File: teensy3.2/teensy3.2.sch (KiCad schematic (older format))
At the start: 80 parts, among them J2 USB_B_Micro, SW1 Prog, U1 LP38691SD-3.3, U2 MKL02Z32VFG4, U3 MK20DX256VLH7, Y1 32.768 KHz, Y2 16 MHz

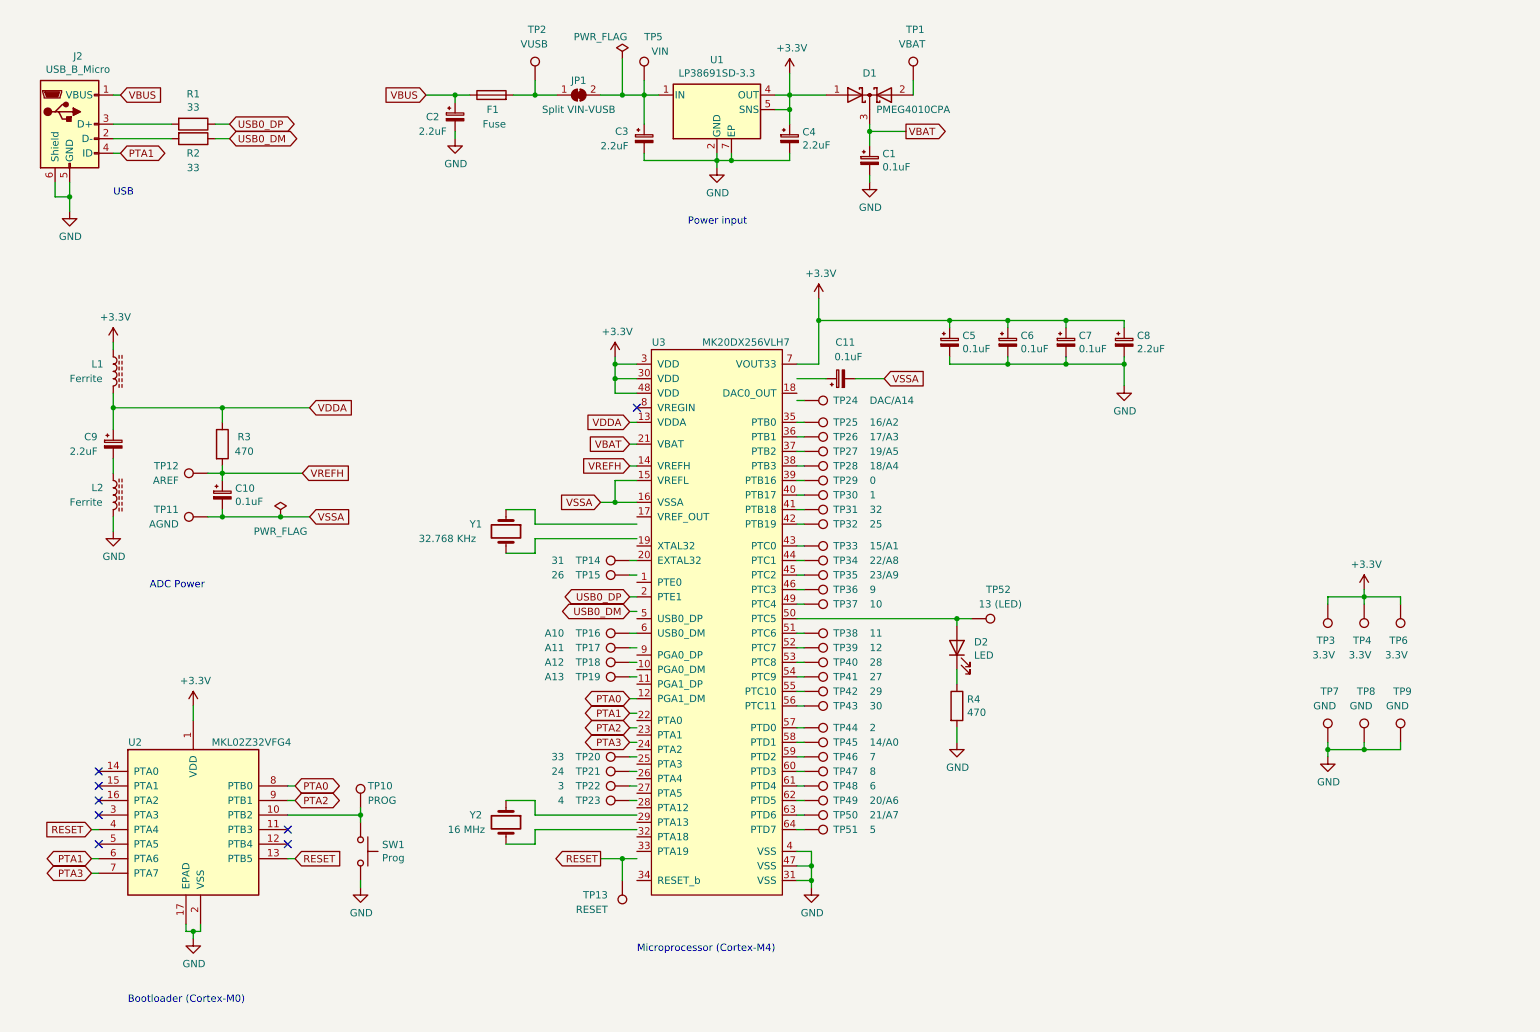
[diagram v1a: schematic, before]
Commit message: avances sch + pcb
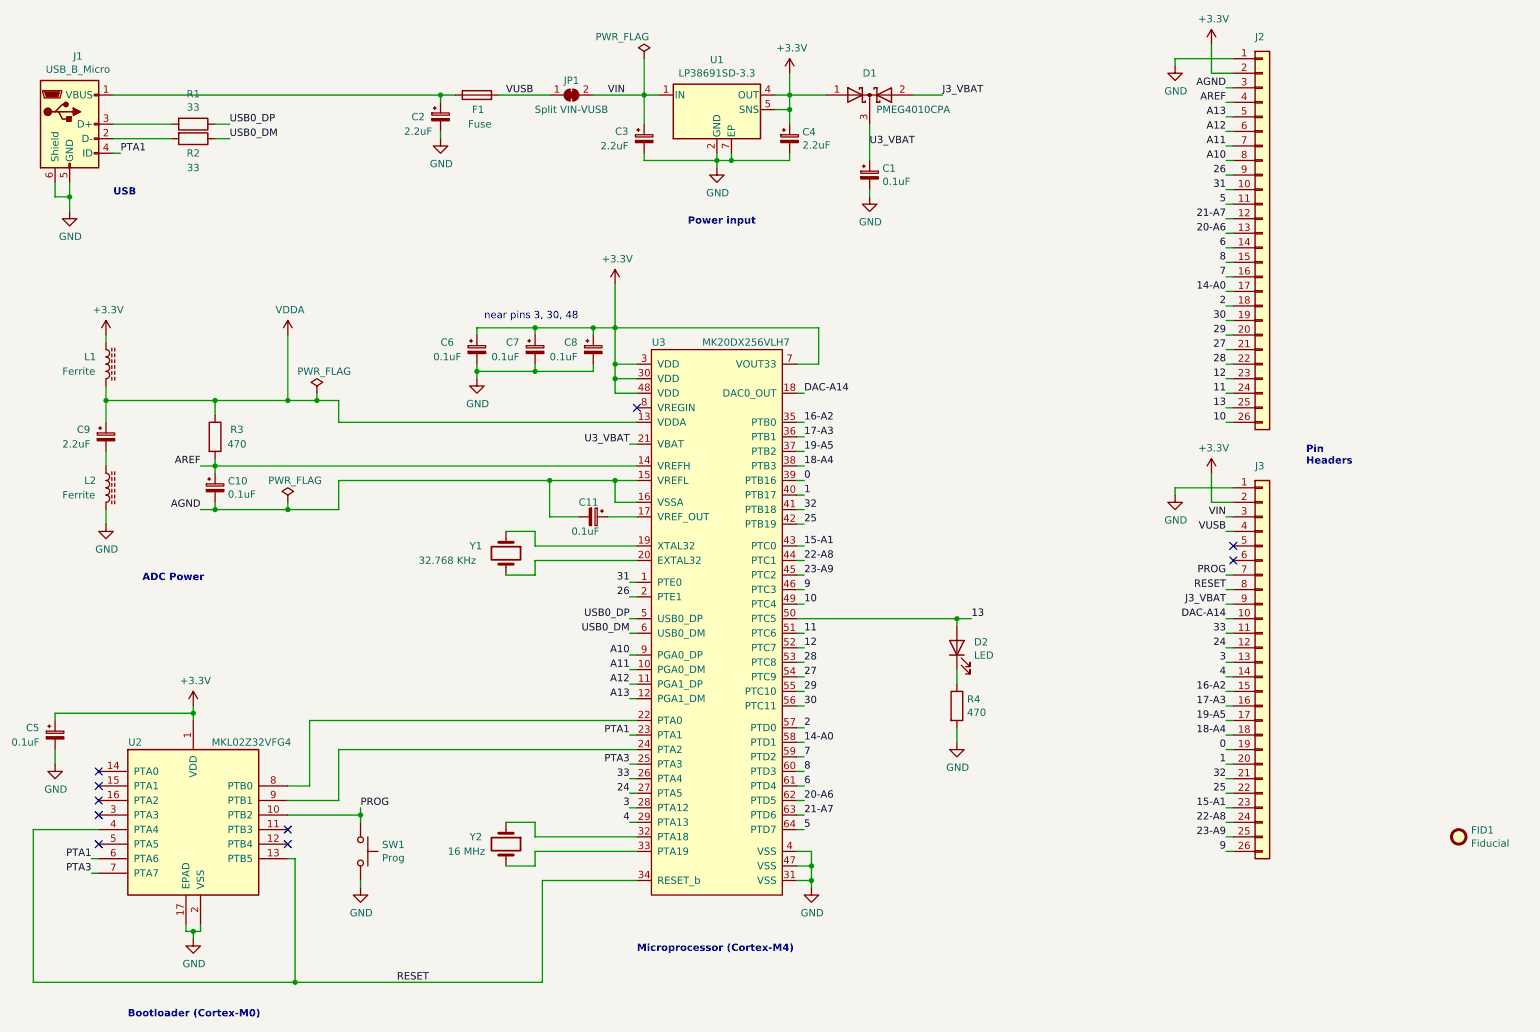
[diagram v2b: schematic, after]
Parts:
- removed TP1: VBAT, TestPoint:TestPoint_THTPad_D2.0mm_Drill1.0mm, symbol Connector:TestPoint
- removed TP10: PROG, TestPoint:TestPoint_THTPad_D2.0mm_Drill1.0mm, symbol Connector:TestPoint
- removed TP11: AGND, TestPoint:TestPoint_THTPad_D2.0mm_Drill1.0mm, symbol Connector:TestPoint
- removed TP12: AREF, TestPoint:TestPoint_THTPad_D2.0mm_Drill1.0mm, symbol Connector:TestPoint
- removed TP13: RESET, TestPoint:TestPoint_THTPad_D2.0mm_Drill1.0mm, symbol Connector:TestPoint
- removed TP14: 31, TestPoint:TestPoint_THTPad_D2.0mm_Drill1.0mm, symbol Connector:TestPoint
- removed TP15: 26, TestPoint:TestPoint_THTPad_D2.0mm_Drill1.0mm, symbol Connector:TestPoint
- removed TP16: A10, TestPoint:TestPoint_THTPad_D2.0mm_Drill1.0mm, symbol Connector:TestPoint
- removed TP17: A11, TestPoint:TestPoint_THTPad_D2.0mm_Drill1.0mm, symbol Connector:TestPoint
- removed TP18: A12, TestPoint:TestPoint_THTPad_D2.0mm_Drill1.0mm, symbol Connector:TestPoint
- removed TP19: A13, TestPoint:TestPoint_THTPad_D2.0mm_Drill1.0mm, symbol Connector:TestPoint
- removed TP2: VUSB, TestPoint:TestPoint_THTPad_D2.0mm_Drill1.0mm, symbol Connector:TestPoint
- removed TP20: 33, TestPoint:TestPoint_THTPad_D2.0mm_Drill1.0mm, symbol Connector:TestPoint
- removed TP21: 24, TestPoint:TestPoint_THTPad_D2.0mm_Drill1.0mm, symbol Connector:TestPoint
- removed TP22: 3, TestPoint:TestPoint_THTPad_D2.0mm_Drill1.0mm, symbol Connector:TestPoint
- removed TP23: 4, TestPoint:TestPoint_THTPad_D2.0mm_Drill1.0mm, symbol Connector:TestPoint
- removed TP24: DAC/A14, TestPoint:TestPoint_THTPad_D2.0mm_Drill1.0mm, symbol Connector:TestPoint
- removed TP25: 16/A2, TestPoint:TestPoint_THTPad_D2.0mm_Drill1.0mm, symbol Connector:TestPoint
- removed TP26: 17/A3, TestPoint:TestPoint_THTPad_D2.0mm_Drill1.0mm, symbol Connector:TestPoint
- removed TP27: 19/A5, TestPoint:TestPoint_THTPad_D2.0mm_Drill1.0mm, symbol Connector:TestPoint
- removed TP28: 18/A4, TestPoint:TestPoint_THTPad_D2.0mm_Drill1.0mm, symbol Connector:TestPoint
- removed TP29: 0, TestPoint:TestPoint_THTPad_D2.0mm_Drill1.0mm, symbol Connector:TestPoint
- removed TP3, TP4, TP6: 3.3V, TestPoint:TestPoint_THTPad_D2.0mm_Drill1.0mm, symbol Connector:TestPoint
- removed TP30: 1, TestPoint:TestPoint_THTPad_D2.0mm_Drill1.0mm, symbol Connector:TestPoint
- removed TP31: 32, TestPoint:TestPoint_THTPad_D2.0mm_Drill1.0mm, symbol Connector:TestPoint
- removed TP32: 25, TestPoint:TestPoint_THTPad_D2.0mm_Drill1.0mm, symbol Connector:TestPoint
- removed TP33: 15/A1, TestPoint:TestPoint_THTPad_D2.0mm_Drill1.0mm, symbol Connector:TestPoint
- removed TP34: 22/A8, TestPoint:TestPoint_THTPad_D2.0mm_Drill1.0mm, symbol Connector:TestPoint
- removed TP35: 23/A9, TestPoint:TestPoint_THTPad_D2.0mm_Drill1.0mm, symbol Connector:TestPoint
- removed TP36: 9, TestPoint:TestPoint_THTPad_D2.0mm_Drill1.0mm, symbol Connector:TestPoint
- removed TP37: 10, TestPoint:TestPoint_THTPad_D2.0mm_Drill1.0mm, symbol Connector:TestPoint
- removed TP38: 11, TestPoint:TestPoint_THTPad_D2.0mm_Drill1.0mm, symbol Connector:TestPoint
- removed TP39: 12, TestPoint:TestPoint_THTPad_D2.0mm_Drill1.0mm, symbol Connector:TestPoint
- removed TP40: 28, TestPoint:TestPoint_THTPad_D2.0mm_Drill1.0mm, symbol Connector:TestPoint
- removed TP41: 27, TestPoint:TestPoint_THTPad_D2.0mm_Drill1.0mm, symbol Connector:TestPoint
- removed TP42: 29, TestPoint:TestPoint_THTPad_D2.0mm_Drill1.0mm, symbol Connector:TestPoint
- removed TP43: 30, TestPoint:TestPoint_THTPad_D2.0mm_Drill1.0mm, symbol Connector:TestPoint
- removed TP44: 2, TestPoint:TestPoint_THTPad_D2.0mm_Drill1.0mm, symbol Connector:TestPoint
- removed TP45: 14/A0, TestPoint:TestPoint_THTPad_D2.0mm_Drill1.0mm, symbol Connector:TestPoint
- removed TP46: 7, TestPoint:TestPoint_THTPad_D2.0mm_Drill1.0mm, symbol Connector:TestPoint
- removed TP47: 8, TestPoint:TestPoint_THTPad_D2.0mm_Drill1.0mm, symbol Connector:TestPoint
- removed TP48: 6, TestPoint:TestPoint_THTPad_D2.0mm_Drill1.0mm, symbol Connector:TestPoint
- removed TP49: 20/A6, TestPoint:TestPoint_THTPad_D2.0mm_Drill1.0mm, symbol Connector:TestPoint
- removed TP5: VIN, TestPoint:TestPoint_THTPad_D2.0mm_Drill1.0mm, symbol Connector:TestPoint
- removed TP50: 21/A7, TestPoint:TestPoint_THTPad_D2.0mm_Drill1.0mm, symbol Connector:TestPoint
- removed TP51: 5, TestPoint:TestPoint_THTPad_D2.0mm_Drill1.0mm, symbol Connector:TestPoint
- removed TP52: 13 (LED), TestPoint:TestPoint_THTPad_D2.0mm_Drill1.0mm, symbol Connector:TestPoint
- removed TP7, TP8, TP9: GND, TestPoint:TestPoint_THTPad_D2.0mm_Drill1.0mm, symbol Connector:TestPoint
- added FID1: Fiducial, Fiducial:Fiducial_0.5mm_Mask1.5mm, symbol Mechanical:Fiducial
- added J2, J3: Conn_01x26, Connector_PinSocket_2.54mm:PinSocket_1x26_P2.54mm_Vertical, symbol Connector_Generic:Conn_01x26
- C1, C10, C11, C5, C6, C7: footprint Capacitor_SMD:C_0603_1608Metric -> Capacitor_SMD:C_0805_2012Metric
- C8: value 2.2uF -> 0.1uF
- D1: Digikey# (none) -> 1727-5212-2-ND
- J1: renamed from J2; Digikey# (none) -> 2134441-2
- L1, L2: footprint Inductor_SMD:L_0201_0603Metric -> Inductor_SMD:L_0805_2012Metric; Digikey# (none) -> 2035-0805CS-331EKFSTR-ND
- R1, R2, R3, R4: footprint Resistor_SMD:R_0201_0603Metric -> Resistor_SMD:R_0805_2012Metric
- U1: Digikey# (none) -> LP38691SD-3.3/NOPBTR-ND
- U2: Digikey# (none) -> MKL02Z32VFG4-ND
- U3: Digikey# (none) -> MK20DX256VLH7-ND
- Y1: footprint Crystal:Crystal_SMD_TXC_AX_8045-2Pin_8.0x4.5mm -> Crystal:Crystal_SMD_2012-2Pin_2.0x1.2mm; Digikey# (none) -> XC2743CT-ND
- Y2: footprint Crystal:Crystal_SMD_HC49-SD -> Crystal:Crystal_SMD_2016-4Pin_2.0x1.6mm; Digikey# (none) -> XC2630TR-ND
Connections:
- net labels added: 0, 1, 10, 11, 12, 13, 14-A0, 15-A1, 16-A2, 17-A3, 18-A4, 19-A5, 2, 20-A6, 21-A7, 22-A8, 23-A9, 24, 25, 26, 27, 28, 29, 3, 30, 31, 32, 33, 4, 5, 6, 7, 8, 9, A10, A11, A12, A13, AGND, AREF, DAC-A14, J3_VBAT, PROG, U3_VBAT, VIN, VUSB
- net labels removed: PTA0, PTA2, VBAT, VBUS, VREFH, VSSA
- wire segments 190 -> 239
- no-connect marks 8 -> 10
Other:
- note added: "Pin\nHeaders"
- note added: "near pins 3, 30, 48"
- moved on the sheet: C1, C10, C11, C2, C5, C6, C7, C8, C9, F1, JP1, L1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
